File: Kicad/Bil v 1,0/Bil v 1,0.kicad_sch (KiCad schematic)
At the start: 15 parts, among them J1 Analog, J2 Digital, J3 Lidar_sensor_adafruit_VL53L0X, J4 Lidar_sensor_adafruit_VL53L0X, J5 Conn_01x04, J6 Lidar_sensor_adafruit_VL53L0X, M1 Motor_DC, M2 Motor_Servo, M3 Motor_DC, M4 Motor_DC

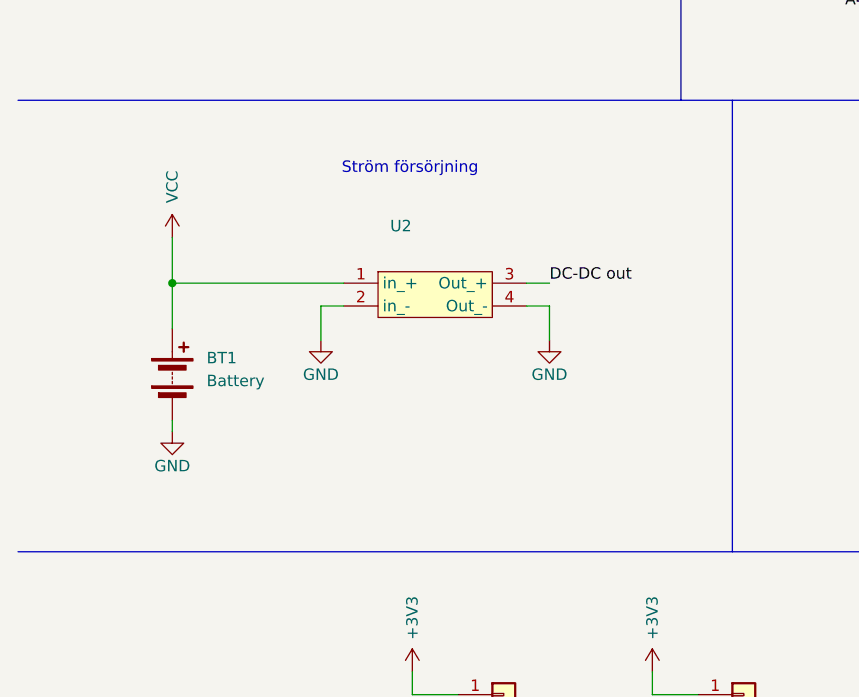
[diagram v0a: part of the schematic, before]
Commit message: 1.3 updated layout
the probably final board layout, now with power switch
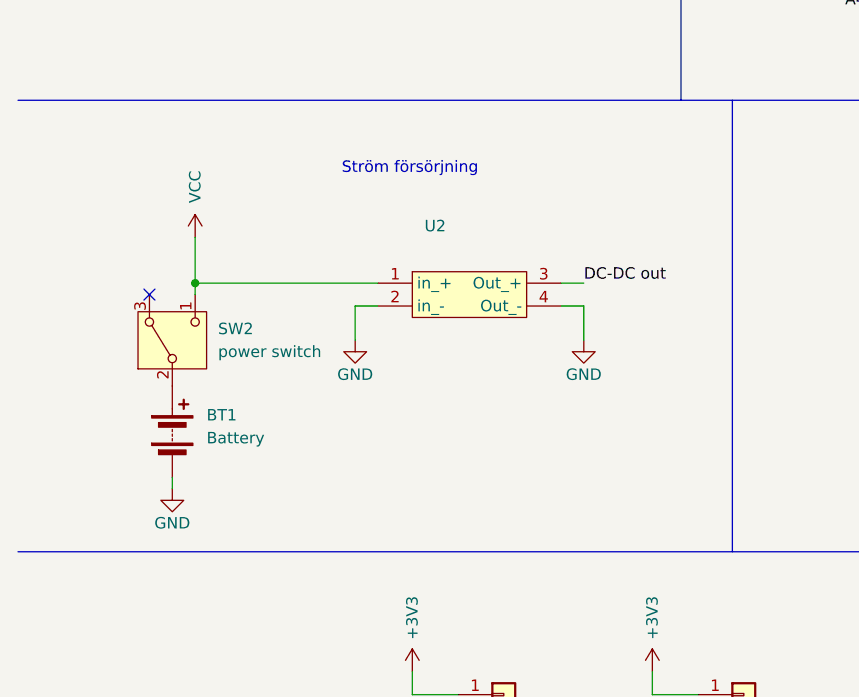
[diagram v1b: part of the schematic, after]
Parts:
- added SW2: power switch, Button_Switch_THT:SW_Slide-03_Wuerth-WS-SLTV_10x2.5x6.4_P2.54mm, symbol Switch:SW_Nidec_CAS-120A1
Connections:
- net VCC: now also SW2.1 (C); no longer BT1.1 (+)
- new net: BT1.1 (+), SW2.2 (B)
- no-connect marks 25 -> 26
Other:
- moved on the sheet: BT1, U2
